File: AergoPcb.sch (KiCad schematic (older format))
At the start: 16 parts, among them J3 Conn_01x04, SW1 SW_Push, U1 ATmega32U4-AU, Y1 16MHz

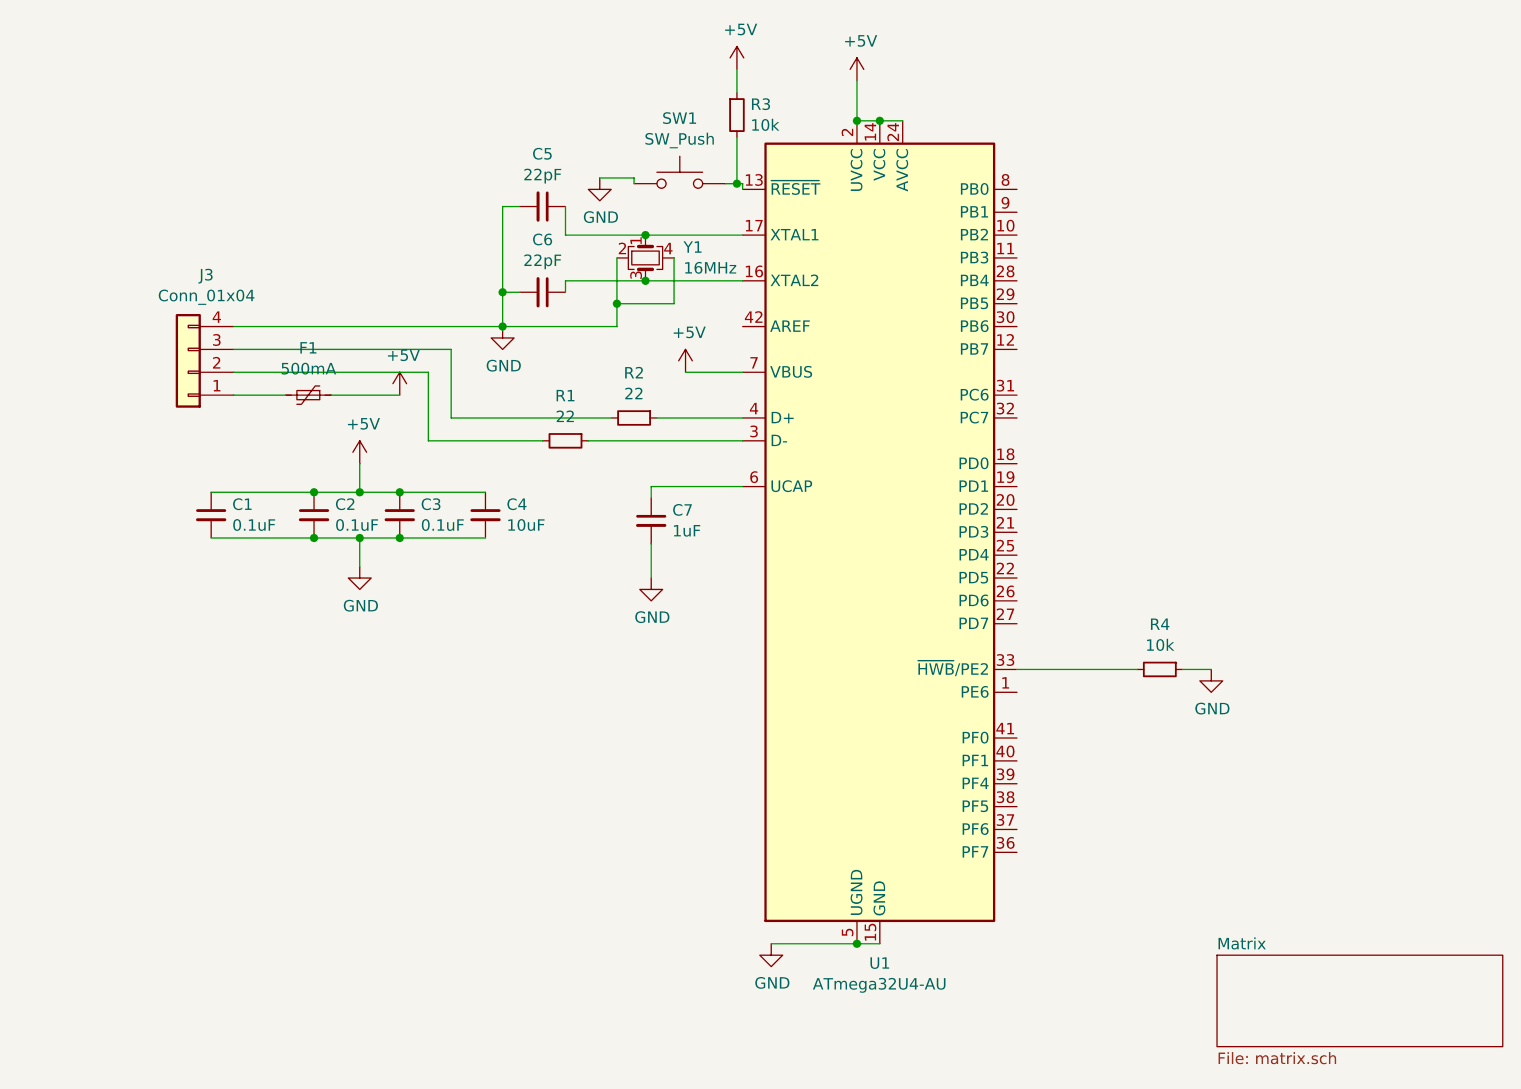
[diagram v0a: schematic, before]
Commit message: Finalized PCB and created Gerbers
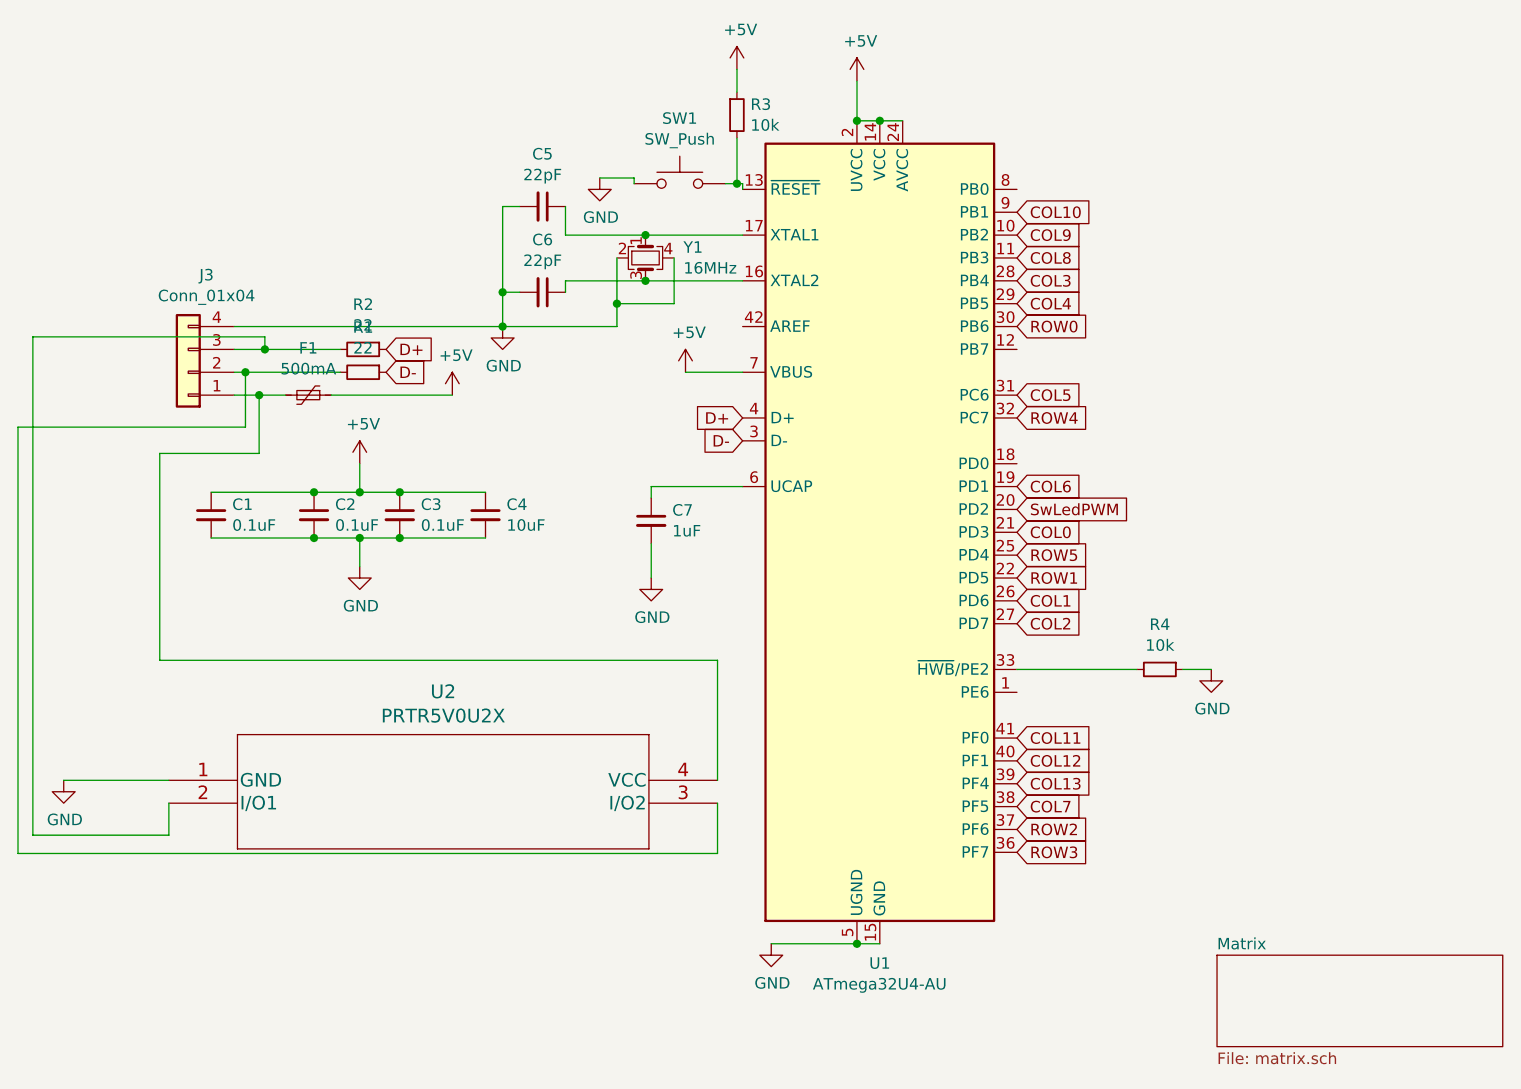
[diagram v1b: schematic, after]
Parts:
- added U2: PRTR5V0U2X, random-keyboard-parts:SOT143B, symbol 2019-04-04_07-10-47:PRTR5V0U2X
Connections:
- net GND: now also U2.1 (GND)
- net COL9: now reaches U1.10 (PB2)
- net COL8: now reaches U1.11 (PB3)
- net COL6: now reaches U1.19 (PD1)
- net SwLedPWM: now reaches U1.20 (PD2)
- net COL0: now reaches U1.21 (PD3)
- net ROW1: now reaches U1.22 (PD5)
- net ROW5: now reaches U1.25 (PD4)
- net COL1: now reaches U1.26 (PD6)
- net COL2: now reaches U1.27 (PD7)
- net COL3: now reaches U1.28 (PB4)
- net COL4: now reaches U1.29 (PB5)
- net D-: now reaches R1.1, U1.3 (D-)
- net ROW0: now reaches U1.30 (PB6)
- net COL5: now reaches U1.31 (PC6)
- net ROW4: now reaches U1.32 (PC7)
- net ROW3: now reaches U1.36 (PF7)
- net ROW2: now reaches U1.37 (PF6)
- net COL7: now reaches U1.38 (PF5)
- net COL13: now reaches U1.39 (PF4)
- net D+: now reaches R2.1, U1.4 (D+)
- net COL12: now reaches U1.40 (PF1)
- net COL11: now reaches U1.41 (PF0)
- net COL10: now reaches U1.9 (PB1)
- net at J3.3 (Pin_3), R2.2: now also U2.2 (I/O1)
- net at J3.2 (Pin_2), R1.2: now also U2.3 (I/O2)
- net at F1.2, J3.1 (Pin_1): now also U2.4 (VCC)
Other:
- moved on the sheet: R1, R2
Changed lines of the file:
@@
 L Device:R_Small R2
 U 1 1 5C80D3A9
-P 3225 3125
-F 0 "R2" V 3029 3125 50  0000 C CNN
-F 1 "22" V 3120 3125 50  0000 C CNN
-F 2 "Resistor_SMD:R_0805_2012Metric" H 3225 3125 50  0001 C CNN
-F 3 "~" H 3225 3125 50  0001 C CNN
-	1    3225 3125
+P 2040 2825
+F 0 "R2" V 1844 2825 50  0000 C CNN
+F 1 "22" V 1935 2825 50  0000 C CNN
+F 2 "Resistor_SMD:R_0805_2012Metric" H 2040 2825 50  0001 C CNN
+F 3 "~" H 2040 2825 50  0001 C CNN
+	1    2040 2825
 	0    1    1    0
 $EndComp
@@
 L Device:R_Small R1
 U 1 1 5C80D430
-P 2925 3225
-F 0 "R1" V 2729 3225 50  0000 C CNN
-F 1 "22" V 2820 3225 50  0000 C CNN
-F 2 "Resistor_SMD:R_0805_2012Metric" H 2925 3225 50  0001 C CNN
-F 3 "~" H 2925 3225 50  0001 C CNN
-	1    2925 3225
-	0    1    1    0
-$EndComp
-Wire Wire Line
-	3700 3225 3025 3225
-Wire Wire Line
-	3700 3125 3325 3125
+P 2040 2925
+F 0 "R1" V 1844 2925 50  0000 C CNN
+F 1 "22" V 1935 2925 50  0000 C CNN
+F 2 "Resistor_SMD:R_0805_2012Metric" H 2040 2925 50  0001 C CNN
+F 3 "~" H 2040 2925 50  0001 C CNN
+	1    2040 2925
+	0    1    1    0
+$EndComp
 $Comp
 L Device:C_Small C7
@@
 $EndComp
 Wire Wire Line
-	2325 3225 2825 3225
-Wire Wire Line
 	3675 1600 3675 1700
-Wire Wire Line
-	2325 3225 2325 2925
-Wire Wire Line
-	2425 3125 2425 2825
-Wire Wire Line
-	2425 3125 3125 3125
 $Comp
 L Device:Polyfuse_Small F1
@@
 	1475 2725 2650 2725
 Wire Wire Line
-	1475 2825 2425 2825
-Wire Wire Line
-	1475 2925 2325 2925
-Wire Wire Line
-	1475 3025 1700 3025
+	1475 3025 1585 3025
 Wire Wire Line
 	2025 3325 2025 3450
@@
 L power:+5V #PWR0101
 U 1 1 5CBAF4D0
-P 2200 3025
-F 0 "#PWR0101" H 2200 2875 50  0001 C CNN
-F 1 "+5V" H 2215 3198 50  0000 C CNN
-F 2 "" H 2200 3025 50  0001 C CNN
-F 3 "" H 2200 3025 50  0001 C CNN
-	1    2200 3025
-	1    0    0    -1
-$EndComp
-Wire Wire Line
-	1900 3025 2200 3025
+P 2430 3025
+F 0 "#PWR0101" H 2430 2875 50  0001 C CNN
+F 1 "+5V" H 2445 3198 50  0000 C CNN
+F 2 "" H 2430 3025 50  0001 C CNN
+F 3 "" H 2430 3025 50  0001 C CNN
+	1    2430 3025
+	1    0    0    -1
+$EndComp
+Text GLabel 4900 2425 2    50   Input ~ 0
+COL8
+Text GLabel 4900 2325 2    50   Input ~ 0
+COL9
+Text GLabel 4900 2225 2    50   Input ~ 0
+COL10
+Text GLabel 4900 4525 2    50   Input ~ 0
+COL11
+Text GLabel 4900 4625 2    50   Input ~ 0
+COL12
+Text GLabel 4900 4725 2    50   Input ~ 0
+COL13
+Text GLabel 4900 4825 2    50   Input ~ 0
+COL7
+Text GLabel 4900 4925 2    50   Input ~ 0
+ROW2
+Text GLabel 4900 5025 2    50   Input ~ 0
+ROW3
+Text GLabel 4900 3725 2    50   Input ~ 0
+ROW5
+Text GLabel 4900 3125 2    50   Input ~ 0
+ROW4
+Text GLabel 4900 3025 2    50   Input ~ 0
+COL5
+Text GLabel 4900 2725 2    50   Input ~ 0
+ROW0
+Text GLabel 4900 3925 2    50   Input ~ 0
+COL1
+Text GLabel 4900 2525 2    50   Input ~ 0
+COL3
+Text GLabel 4900 2625 2    50   Input ~ 0
+COL4
+Text GLabel 4900 4025 2    50   Input ~ 0
+COL2
+Text GLabel 4900 3825 2    50   Input ~ 0
+ROW1
+Text GLabel 4900 3625 2    50   Input ~ 0
+COL0
+Text GLabel 4900 3525 2    50   Input ~ 0
+SwLedPWM
+Text GLabel 4900 3425 2    50   Input ~ 0
+COL6
+$Comp
+L 2019-04-04_07-10-47:PRTR5V0U2X U2
+U 1 1 5CA5BEBF
+P 1190 4710
+F 0 "U2" H 2390 5097 60  0000 C CNN
+F 1 "PRTR5V0U2X" H 2390 4991 60  0000 C CNN
+F 2 "random-keyboard-parts:SOT143B" H 2390 4950 60  0001 C CNN
+F 3 "" H 1190 4710 60  0000 C CNN
+	1    1190 4710
+	1    0    0    -1
+$EndComp
+$Comp
+L power:GND #PWR0102
+U 1 1 5CA5EE38
+P 730 4710
+F 0 "#PWR0102" H 730 4460 50  0001 C CNN
+F 1 "GND" H 735 4537 50  0000 C CNN
+F 2 "" H 730 4710 50  0001 C CNN
+F 3 "" H 730 4710 50  0001 C CNN
+	1    730  4710
+	1    0    0    -1
+$EndComp
+Wire Wire Line
+	1190 4710 730  4710
+Wire Wire Line
+	1475 2925 1525 2925
+Wire Wire Line
+	1475 2825 1610 2825
+Text GLabel 2140 2825 2    50   Input ~ 0
+D+
+Text GLabel 2140 2925 2    50   Input ~ 0
+D-
+Wire Wire Line
+	1900 3025 2430 3025
+Wire Wire Line
+	1585 3025 1585 3280
+Wire Wire Line
+	1585 3280 1150 3280
+Wire Wire Line
+	1150 3280 1150 4185
+Wire Wire Line
+	1150 4185 3590 4185
+Wire Wire Line
+	3590 4185 3590 4710
+Connection ~ 1585 3025
+Wire Wire Line
+	1585 3025 1700 3025
+Text GLabel 3700 3125 0    50   Input ~ 0
+D+
+Text GLabel 3700 3225 0    50   Input ~ 0
+D-
+Wire Wire Line
+	1610 2825 1610 2770
+Wire Wire Line
+	1610 2770 595  2770
+Wire Wire Line
+	595  2770 595  4950
+Wire Wire Line
+	595  4950 1190 4950
+Wire Wire Line
+	1190 4950 1190 4810
+Connection ~ 1610 2825
+Wire Wire Line
+	1610 2825 1940 2825
+Wire Wire Line
+	3590 4810 3590 5030
+Wire Wire Line
+	3590 5030 530  5030
+Wire Wire Line
+	530  5030 530  3165
+Wire Wire Line
+	530  3165 1525 3165
+Wire Wire Line
+	1525 3165 1525 2925
+Connection ~ 1525 2925
+Wire Wire Line
+	1525 2925 1940 2925
 $EndSCHEMATC
